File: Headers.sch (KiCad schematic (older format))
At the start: 1 part

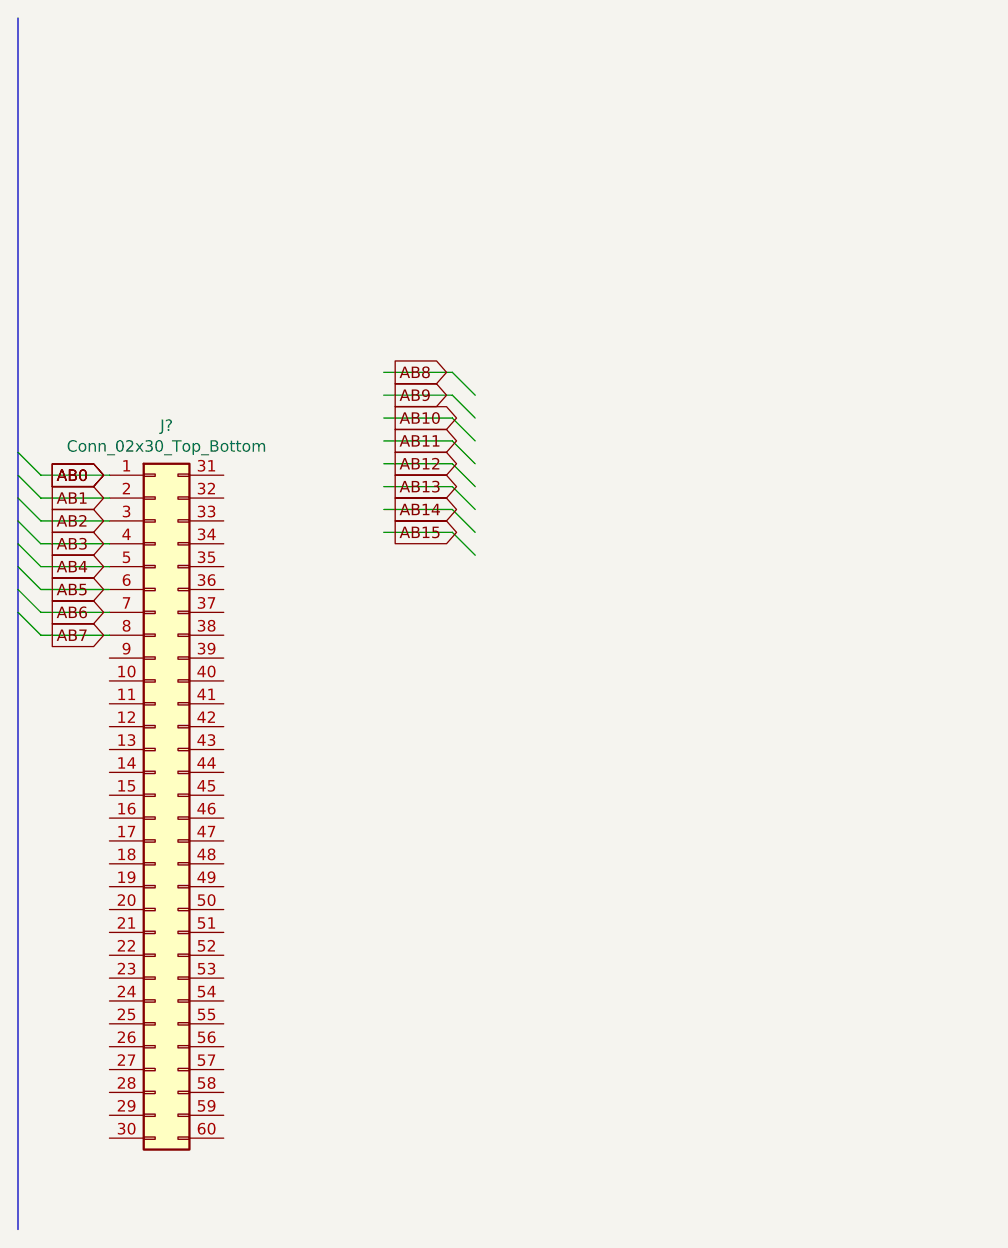
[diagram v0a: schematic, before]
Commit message: sram v1
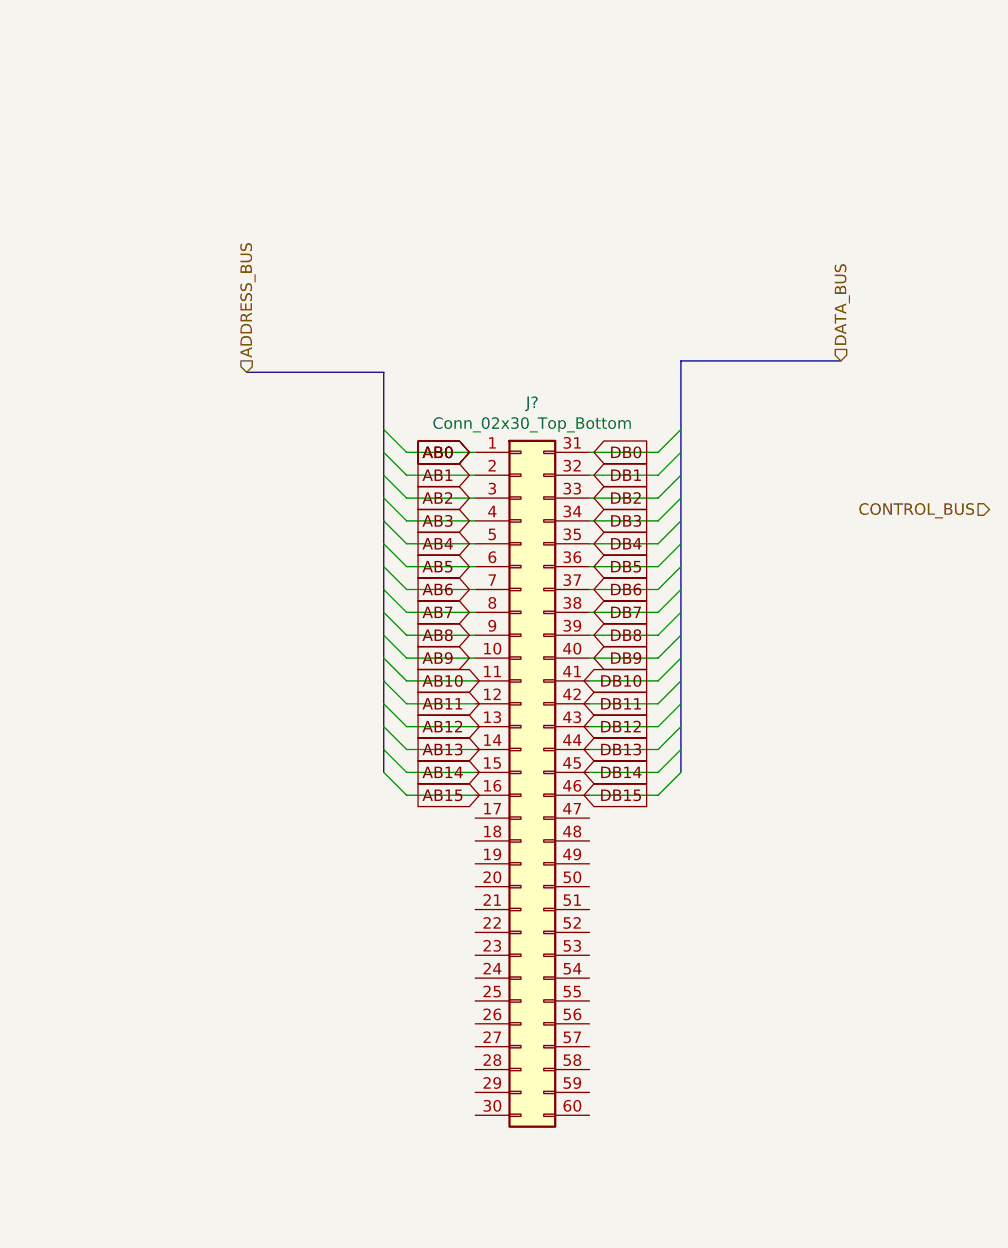
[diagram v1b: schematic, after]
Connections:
- net labels added: ADDRESS_BUS, CONTROL_BUS, DATA_BUS, DB0, DB1, DB10, DB11, DB12, DB13, DB14, DB15, DB2, DB3, DB4, DB5, DB6, DB7, DB8, DB9
- wire segments 16 -> 32
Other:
- moved on the sheet: J?
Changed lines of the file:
@@
 $Descr A4 11693 8268
 encoding utf-8
-Sheet 5 7
+Sheet 3 8
 Title ""
 Date ""
@@
 L Connector_Generic:Conn_02x30_Top_Bottom J?
 U 1 1 5EA32CD9
-P 2200 4550
-F 0 "J?" H 2250 6167 50  0000 C CNN
-F 1 "Conn_02x30_Top_Bottom" H 2250 6076 50  0000 C CNN
-F 2 "" H 2200 4550 50  0001 C CNN
-F 3 "~" H 2200 4550 50  0001 C CNN
-	1    2200 4550
+P 3800 4450
+F 0 "J?" H 3850 6067 50  0000 C CNN
+F 1 "Conn_02x30_Top_Bottom" H 3850 5976 50  0000 C CNN
+F 2 "" H 3800 4450 50  0001 C CNN
+F 3 "~" H 3800 4450 50  0001 C CNN
+	1    3800 4450
 	1    0    0    -1
 $EndComp
 Entry Wire Line
-	1700 3850 1600 3750
-Entry Wire Line
-	1700 3750 1600 3650
-Entry Wire Line
-	1700 3650 1600 3550
-Entry Wire Line
-	1700 3550 1600 3450
-Entry Wire Line
-	1700 3450 1600 3350
-Entry Wire Line
-	1700 3350 1600 3250
-Entry Wire Line
-	1700 3250 1600 3150
-Entry Wire Line
-	1700 3150 1600 3050
-Entry Wire Line
-	3500 2700 3600 2800
-Entry Wire Line
-	3500 2800 3600 2900
-Entry Wire Line
-	3500 2900 3600 3000
-Entry Wire Line
-	3500 3000 3600 3100
-Entry Wire Line
-	3500 3100 3600 3200
-Entry Wire Line
-	3500 3200 3600 3300
-Entry Wire Line
-	3500 3300 3600 3400
-Entry Wire Line
-	3500 3400 3600 3500
-Text GLabel 1750 3150 2    50   Output ~ 0
+	3300 3750 3200 3650
+Entry Wire Line
+	3300 3650 3200 3550
+Entry Wire Line
+	3300 3550 3200 3450
+Entry Wire Line
+	3300 3450 3200 3350
+Entry Wire Line
+	3300 3350 3200 3250
+Entry Wire Line
+	3300 3250 3200 3150
+Entry Wire Line
+	3300 3150 3200 3050
+Entry Wire Line
+	3300 3050 3200 2950
+Text GLabel 3350 3050 2    50   Output ~ 0
 AB0
-Text GLabel 1750 3250 2    50   Output ~ 0
+Text GLabel 3350 3150 2    50   Output ~ 0
 AB1
-Text GLabel 1750 3350 2    50   Output ~ 0
+Text GLabel 3350 3250 2    50   Output ~ 0
 AB2
-Text GLabel 1750 3450 2    50   Output ~ 0
+Text GLabel 3350 3350 2    50   Output ~ 0
 AB3
-Text GLabel 1750 3550 2    50   Output ~ 0
+Text GLabel 3350 3450 2    50   Output ~ 0
 AB4
-Text GLabel 1750 3750 2    50   Output ~ 0
+Text GLabel 3350 3650 2    50   Output ~ 0
 AB6
-Text GLabel 1750 3850 2    50   Output ~ 0
+Text GLabel 3350 3750 2    50   Output ~ 0
 AB7
-Text GLabel 3250 2700 2    50   Output ~ 0
+Text GLabel 3350 3550 2    50   Output ~ 0
+AB5
+Text GLabel 3350 3050 2    50   Output ~ 0
+AB0
+Wire Wire Line
+	3300 3750 3600 3750
+Wire Wire Line
+	3300 3650 3600 3650
+Wire Wire Line
+	3300 3550 3600 3550
+Wire Wire Line
+	3300 3450 3600 3450
+Wire Wire Line
+	3300 3350 3600 3350
+Wire Wire Line
+	3300 3250 3600 3250
+Wire Wire Line
+	3300 3150 3600 3150
+Wire Wire Line
+	3300 3050 3600 3050
+Text GLabel 3350 4550 2    50   Output ~ 0
+AB15
+Text GLabel 3350 4450 2    50   Output ~ 0
+AB14
+Text GLabel 3350 4350 2    50   Output ~ 0
+AB13
+Text GLabel 3350 4250 2    50   Output ~ 0
+AB12
+Wire Wire Line
+	3300 4150 3600 4150
+Wire Wire Line
+	3300 4550 3600 4550
+Wire Wire Line
+	3300 4450 3600 4450
+Wire Wire Line
+	3300 4350 3600 4350
+Wire Wire Line
+	3300 4250 3600 4250
+Wire Wire Line
+	3300 4050 3600 4050
+Wire Wire Line
+	3300 3950 3600 3950
+Wire Wire Line
+	3300 3850 3600 3850
+Text GLabel 3350 4150 2    50   Output ~ 0
+AB11
+Text GLabel 3350 4050 2    50   Output ~ 0
+AB10
+Text GLabel 3350 3950 2    50   Output ~ 0
+AB9
+Text GLabel 3350 3850 2    50   Output ~ 0
 AB8
-Text GLabel 3250 2800 2    50   Output ~ 0
-AB9
-Text GLabel 3250 2900 2    50   Output ~ 0
-AB10
-Text GLabel 3250 3000 2    50   Output ~ 0
-AB11
-Text GLabel 1750 3650 2    50   Output ~ 0
-AB5
-Wire Wire Line
-	3200 2700 3500 2700
-Wire Wire Line
-	3200 2800 3500 2800
-Wire Wire Line
-	3200 2900 3500 2900
-Wire Wire Line
-	3200 3100 3500 3100
-Wire Wire Line
-	3200 3200 3500 3200
-Wire Wire Line
-	3200 3300 3500 3300
-Wire Wire Line
-	3200 3400 3500 3400
-Wire Wire Line
-	3200 3000 3500 3000
-Text GLabel 3250 3100 2    50   Output ~ 0
-AB12
-Text GLabel 3250 3200 2    50   Output ~ 0
-AB13
-Text GLabel 3250 3300 2    50   Output ~ 0
-AB14
-Text GLabel 3250 3400 2    50   Output ~ 0
-AB15
-Text GLabel 1750 3150 2    50   Output ~ 0
-AB0
-Wire Wire Line
-	1700 3850 2000 3850
-Wire Wire Line
-	1700 3750 2000 3750
-Wire Wire Line
-	1700 3650 2000 3650
-Wire Wire Line
-	1700 3550 2000 3550
-Wire Wire Line
-	1700 3450 2000 3450
-Wire Wire Line
-	1700 3350 2000 3350
-Wire Wire Line
-	1700 3250 2000 3250
-Wire Wire Line
-	1700 3150 2000 3150
-Wire Bus Line
-	1600 1150 1600 6450
+Entry Wire Line
+	3300 3850 3200 3750
+Entry Wire Line
+	3300 3950 3200 3850
+Entry Wire Line
+	3300 4050 3200 3950
+Entry Wire Line
+	3300 4150 3200 4050
+Entry Wire Line
+	3300 4250 3200 4150
+Entry Wire Line
+	3300 4350 3200 4250
+Entry Wire Line
+	3300 4450 3200 4350
+Entry Wire Line
+	3300 4550 3200 4450
+Wire Bus Line
+	3200 2700 2600 2700
+Text HLabel 2600 2700 1    50   Input ~ 0
+ADDRESS_BUS
+Entry Wire Line
+	4400 4550 4500 4450
+Entry Wire Line
+	4400 4450 4500 4350
+Entry Wire Line
+	4400 4350 4500 4250
+Entry Wire Line
+	4400 4250 4500 4150
+Entry Wire Line
+	4400 4150 4500 4050
+Entry Wire Line
+	4400 4050 4500 3950
+Text HLabel 5200 2650 1    50   Input ~ 0
+DATA_BUS
+Entry Wire Line
+	4400 3650 4500 3550
+Entry Wire Line
+	4400 3550 4500 3450
+Entry Wire Line
+	4400 3450 4500 3350
+Entry Wire Line
+	4400 3350 4500 3250
+Entry Wire Line
+	4400 3250 4500 3150
+Entry Wire Line
+	4400 3150 4500 3050
+Entry Wire Line
+	4400 3850 4500 3750
+Entry Wire Line
+	4400 3950 4500 3850
+Wire Wire Line
+	4400 4050 4100 4050
+Wire Wire Line
+	4400 4450 4100 4450
+Wire Wire Line
+	4400 4350 4100 4350
+Wire Wire Line
+	4400 4250 4100 4250
+Wire Wire Line
+	4400 4150 4100 4150
+Wire Wire Line
+	4400 3950 4100 3950
+Wire Wire Line
+	4400 4550 4100 4550
+Text GLabel 4350 4050 0    50   Output ~ 0
+DB10
+Text GLabel 4350 3950 0    50   Output ~ 0
+DB9
+Text GLabel 4350 4150 0    50   Output ~ 0
+DB11
+Text GLabel 4350 4250 0    50   Output ~ 0
+DB12
+Text GLabel 4350 4350 0    50   Output ~ 0
+DB13
+Text GLabel 4350 4450 0    50   Output ~ 0
+DB14
+Text GLabel 4350 4550 0    50   Output ~ 0
+DB15
+Entry Wire Line
+	4400 3750 4500 3650
+Entry Wire Line
+	4400 3050 4500 2950
+Wire Wire Line
+	4400 3850 4100 3850
+Text GLabel 4350 3850 0    50   Output ~ 0
+DB8
+Text GLabel 4350 3050 0    50   Output ~ 0
+DB0
+Wire Wire Line
+	4400 3050 4100 3050
+Text GLabel 4350 3650 0    50   Output ~ 0
+DB6
+Text GLabel 4350 3550 0    50   Output ~ 0
+DB5
+Text GLabel 4350 3450 0    50   Output ~ 0
+DB4
+Text GLabel 4350 3350 0    50   Output ~ 0
+DB3
+Text GLabel 4350 3250 0    50   Output ~ 0
+DB2
+Text GLabel 4350 3150 0    50   Output ~ 0
+DB1
+Wire Wire Line
+	4400 3650 4100 3650
+Wire Wire Line
+	4400 3550 4100 3550
+Wire Wire Line
+	4400 3450 4100 3450
+Wire Wire Line
+	4400 3350 4100 3350
+Wire Wire Line
+	4400 3250 4100 3250
+Wire Wire Line
+	4400 3150 4100 3150
+Text GLabel 4350 3750 0    50   Output ~ 0
+DB7
+Wire Wire Line
+	4400 3750 4100 3750
+Wire Bus Line
+	4500 2650 5200 2650
+Wire Bus Line
+	3200 2700 3200 4450
+Wire Bus Line
+	4500 2650 4500 4450
+Text HLabel 5850 3300 0    50   Input ~ 0
+CONTROL_BUS
 $EndSCHEMATC
